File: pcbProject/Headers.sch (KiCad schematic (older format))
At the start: 4 parts, among them P1 Power Header, P2 Analog Header (AD), P3 Digital Header 02 (IOH), P4 Digital Header 01 (IOL)

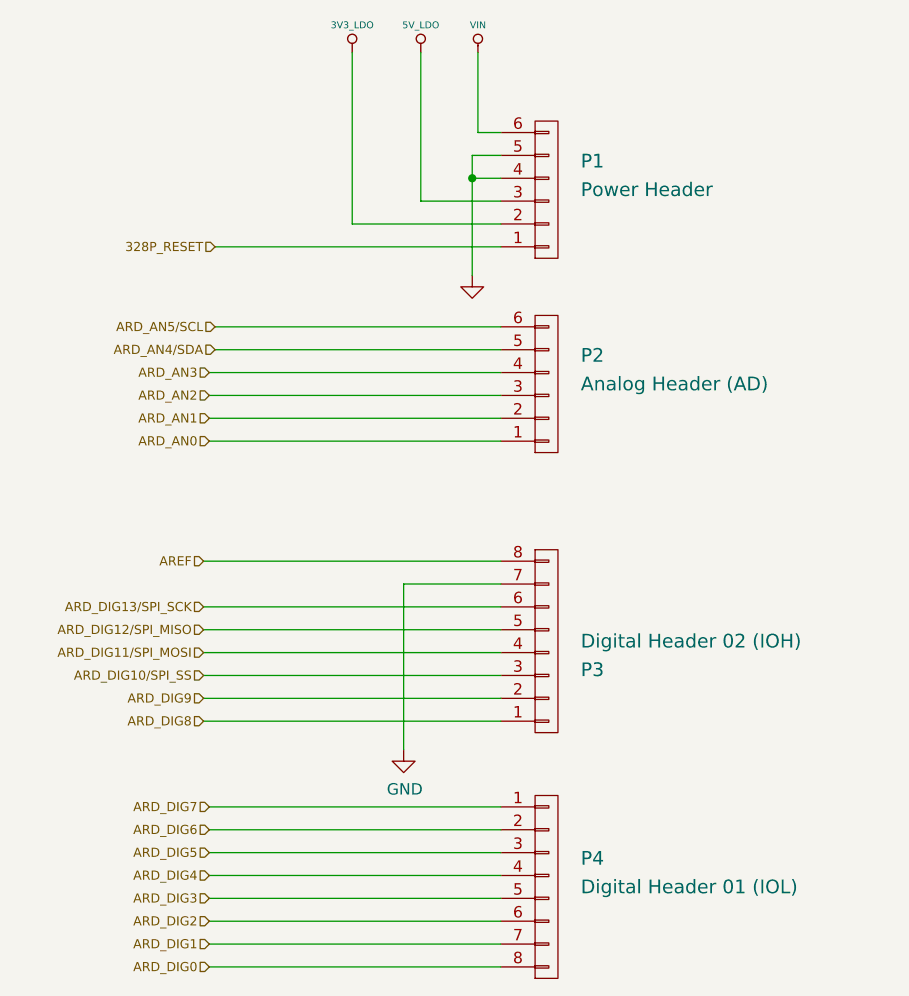
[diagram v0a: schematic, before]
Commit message: schema Afgewerkt
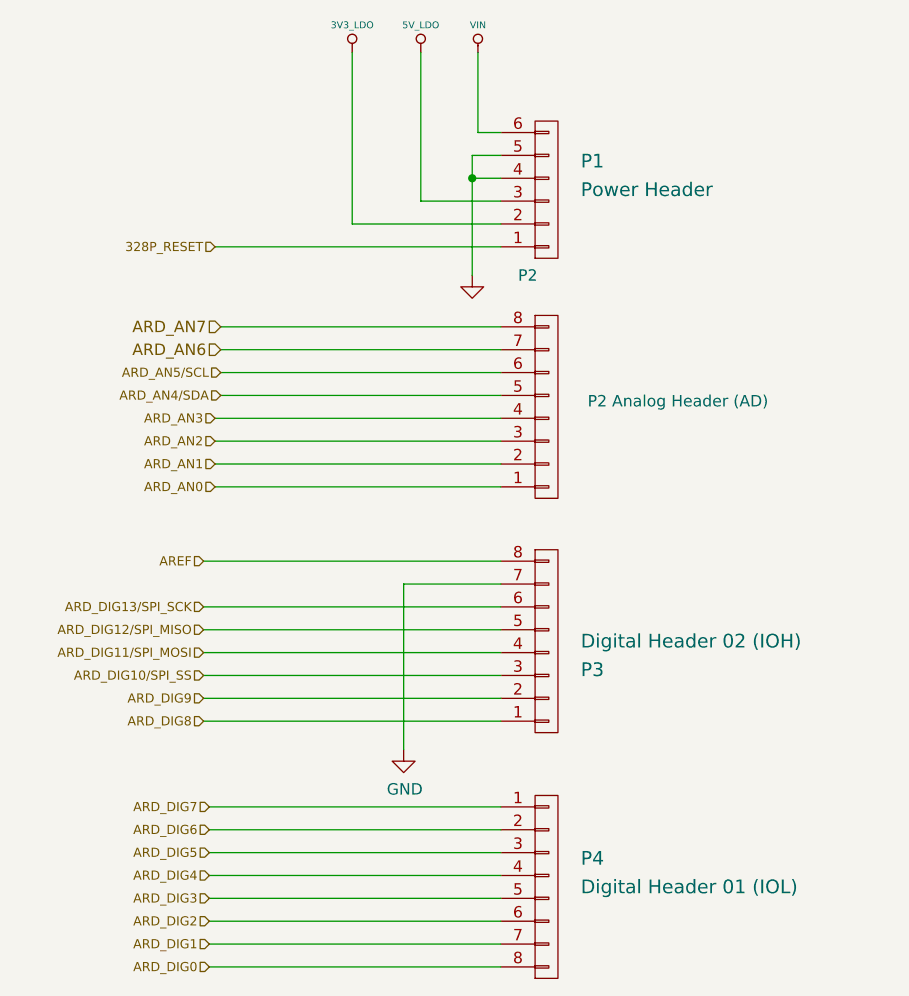
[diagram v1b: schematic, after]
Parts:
- removed P2: Analog Header (AD), ~, symbol Arduino_Uno_R3_From_Scratch-rescue:CONN_01X06
- added P2: P2 Analog Header (AD), symbol Arduino_Uno_R3_From_Scratch-rescue:CONN_01X08
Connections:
- net ARD_AN0: now also P2.1 (P1)
- net ARD_AN1: now also P2.2 (P2)
- net ARD_AN2: now also P2.3 (P3)
- net ARD_AN3: now also P2.4 (P4)
- net ARD_AN4/SDA: now also P2.5 (P5)
- net ARD_AN5/SCL: now also P2.6 (P6)
- new net ARD_AN6: P2.7 (P7)
- new net ARD_AN7: P2.8 (P8)
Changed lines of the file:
@@
 $EndDescr
-$Comp
-L Arduino_Uno_R3_From_Scratch-rescue:CONN_01X06 P2
-U 1 1 55E94764
-P 6250 3325
-F 0 "P2" H 6400 3200 60  0000 L CNN
-F 1 "Analog Header (AD)" H 6400 3325 60  0000 L CNN
-F 2 "~" H 6250 3325 60  0000 C CNN
-F 3 "http://sullinscorp.com/catalogs/101_PAGE114-115_.100_FEMALE_HDR.pdf" H 6250 3325 60  0001 C CNN
-F 4 "Connector Header 6 Position 0.100\" (2.54mm) Gold Surface Mount" H 6250 3325 60  0001 C CNN "Characteristics"
-F 5 "Shield Header 6POS - ANLG" H 6250 3325 60  0001 C CNN "Description"
-F 6 "Sullins Connector" H 6250 3325 60  0001 C CNN "MFN"
-F 7 "NPPC061KFXC-RC" H 6250 3325 60  0001 C CNN "MFP"
-F 8 "SMD" H 6250 3325 60  0001 C CNN "Package ID"
-F 9 "ANY" H 6250 3325 60  0001 C CNN "Source"
-F 10 "N" H 6250 3325 60  0001 C CNN "Critical"
-F 11 "Shield_Headers" H 6250 3325 60  0001 C CNN "Subsystem"
-F 12 "~" H 6250 3325 60  0001 C CNN "Notes"
-	1    6250 3325
-	1    0    0    1
-$EndComp
 $Comp
 L Arduino_Uno_R3_From_Scratch:5V_LDO #PWR035
@@
 Text HLabel 4800 2725 0    40   Input ~ 0
 328P_RESET
-Text HLabel 4775 3275 0    40   Input ~ 0
+Text HLabel 4800 3475 0    40   Input ~ 0
 ARD_AN3
-Text HLabel 4775 3375 0    40   Input ~ 0
+Text HLabel 4800 3575 0    40   Input ~ 0
 ARD_AN2
-Text HLabel 4775 3475 0    40   Input ~ 0
+Text HLabel 4800 3675 0    40   Input ~ 0
 ARD_AN1
-Text HLabel 4775 3575 0    40   Input ~ 0
+Text HLabel 4800 3775 0    40   Input ~ 0
 ARD_AN0
-Wire Wire Line
-	4775 3575 6050 3575
-Wire Wire Line
-	6050 3475 4775 3475
-Wire Wire Line
-	4775 3375 6050 3375
-Wire Wire Line
-	6050 3275 4775 3275
 Text HLabel 4775 5175 0    40   Input ~ 0
 ARD_DIG7
@@
 	1    0    0    -1
 $EndComp
-Text HLabel 4800 3175 0    40   Input ~ 0
+Text HLabel 4825 3375 0    40   Input ~ 0
 ARD_AN4/SDA
-Text HLabel 4800 3075 0    40   Input ~ 0
+Text HLabel 4825 3275 0    40   Input ~ 0
 ARD_AN5/SCL
-Wire Wire Line
-	4800 3075 6050 3075
-Wire Wire Line
-	4800 3175 6050 3175
 Text HLabel 4750 4800 0    40   Input ~ 0
 ARD_DIG8
@@
 Wire Wire Line
 	6050 4700 4750 4700
+$Comp
+L Arduino_Uno_R3_From_Scratch-rescue:CONN_01X08 P2
+U 1 1 5C79CCDA
+P 6250 3425
+F 0 "P2" H 6168 2850 50  0000 C CNN
+F 1 "P2 Analog Header (AD)" H 6825 3400 50  0000 C CNN
+F 2 "" H 6250 3425 60  0000 C CNN
+F 3 "" H 6250 3425 60  0000 C CNN
+	1    6250 3425
+	1    0    0    1
+$EndComp
+Wire Wire Line
+	4800 3775 6050 3775
+Wire Wire Line
+	4800 3675 6050 3675
+Wire Wire Line
+	4800 3575 6050 3575
+Wire Wire Line
+	4800 3475 6050 3475
+Wire Wire Line
+	4825 3375 6050 3375
+Wire Wire Line
+	4825 3275 6050 3275
+Text HLabel 4825 3175 0    50   Input ~ 0
+ARD_AN6
+Text HLabel 4825 3075 0    50   Input ~ 0
+ARD_AN7
+Wire Wire Line
+	4825 3175 6050 3175
+Wire Wire Line
+	4825 3075 6050 3075
 $EndSCHEMATC
